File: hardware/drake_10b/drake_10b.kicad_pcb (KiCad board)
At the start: 4 copper layers, 47.9 x 47.9 mm, 173 parts, among them J1 Conn_02x02_Odd_Even, J10 Conn_01x04, J2 USB_C_Receptacle_USB2.0_16P, J3 Li-Ion, J4 Conn_01x01, J5 Conn_01x04, J6 Conn_01x04, J7 Conn_01x01, J8 Conn_01x04, J9 Conn_01x04, SW1 SW_Push, SW2 SW_Push, SW3 SW_Push, SW4 SW_Push, U1 nRF52832-QFxx, U2 XC6206P332MR-G, U3 TP4054, U4 LIS2DH12TR, U5 BDR6125, U6 ITR8307-S18-TR8, Y1 Crystal_GND24

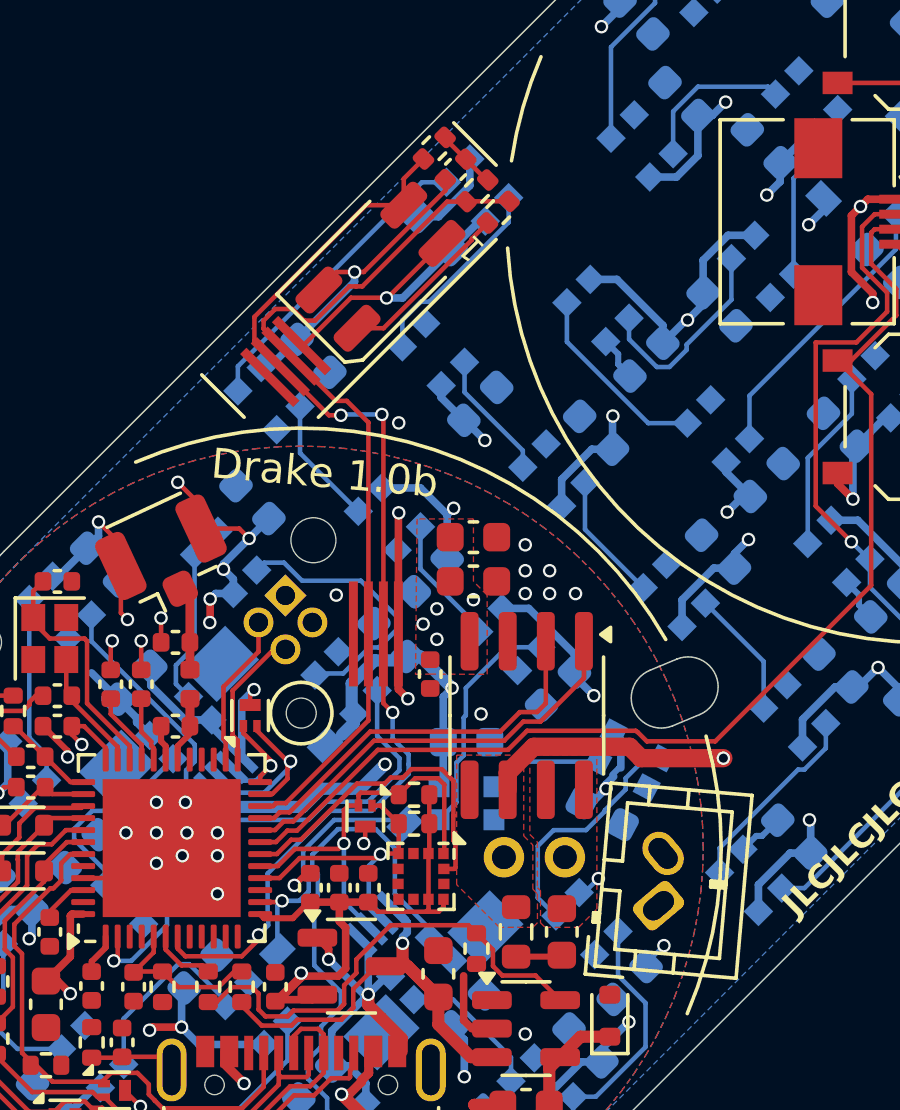
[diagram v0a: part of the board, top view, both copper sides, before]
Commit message: revised production files
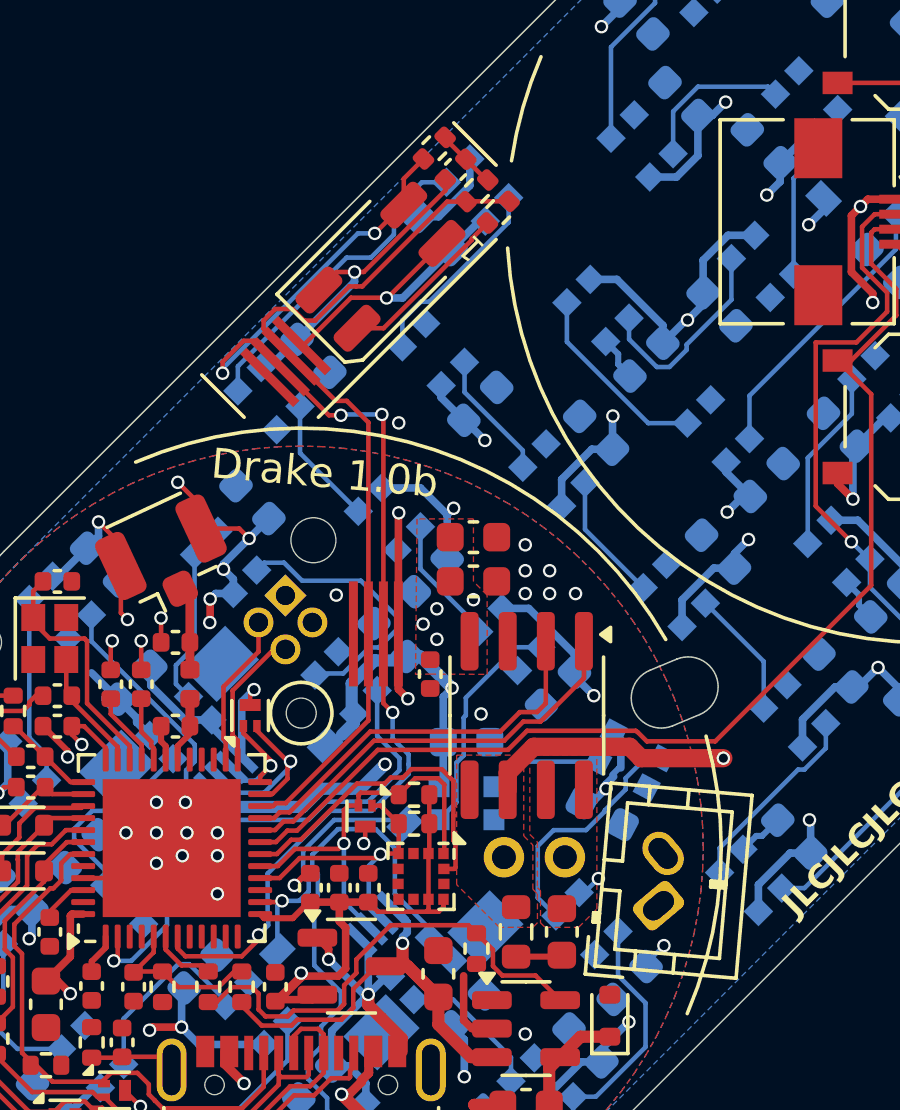
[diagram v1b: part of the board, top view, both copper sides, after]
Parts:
- C68: footprint Capacitor_SMD:C_0402_1005Metric -> Library:C_0402_1005Metric
- D5: value green -> yellow
- D6: value blue -> white
- J10: footprint rt_connectors:FFC_SolderCon_4pin_3,5x0,3mm_Pitch0.5mm -> Library:FFC_SolderCon_4pin_3,5x0,3mm_Pitch0.5mm
- R13: value 82k -> 75k; footprint Resistor_SMD:R_0402_1005Metric -> Library:R_0402_1005Metric
- R14, R18: footprint Resistor_SMD:R_0402_1005Metric -> Library:R_0402_1005Metric
- R15: value 1k5 -> 3k3
- R16: value 470 -> 3k3
- R17: value 220 -> 1k5
- U5: footprint Package_SO:SOIC-8_3.9x4.9mm_P1.27mm -> Library:SOIC-8_3.9x4.9mm_P1.27mm
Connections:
- net /LED_GREEN renamed /LED_YELLOW
- net /LED_RED renamed /LED_WHITE
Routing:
- net /MT_SEN_RET: track 38.6 -> 41.5 mm, vias 4 -> 6
